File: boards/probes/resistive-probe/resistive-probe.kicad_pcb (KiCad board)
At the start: 2 copper layers, 60.5 x 6 mm, 13 parts, among them P1 MMCX, P2 SOLDERPAD, P3 SOLDERPAD

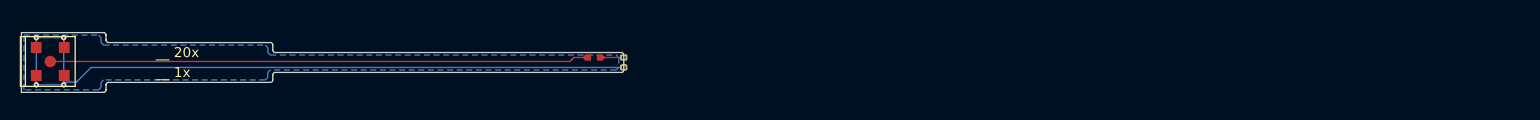
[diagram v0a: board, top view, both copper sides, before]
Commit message: v0.3 AKL-PT2 layout
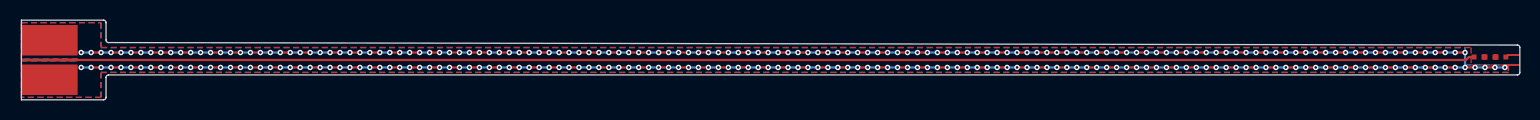
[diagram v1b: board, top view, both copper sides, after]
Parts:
- removed G*** (x4): TEARDROP_03, azonenberg_pcb:TEARDROP_03
- removed G*** (x4): TEARDROP_02, azonenberg_pcb:TEARDROP_02
- removed G***: LOGO, w_logo:Logo_silk_ROHS_5x2.8mm
- removed P1: MMCX, azonenberg_pcb:CONN_MMCX_LINX_CONNMMCX002SMD
- removed P2, P3: SOLDERPAD, azonenberg_pcb:FLEX_SOLDERPAD
- added J1: SMA, azonenberg_pcb:CONN_SMA_EDGE_AMPHENOL_901_10511_3, F.Cu at (89.3, 50.2)
- added J2: TIP, azonenberg_pcb:TESTPOINT_BARETRACE_150UM, F.Cu at (236.4, 49.8)
- added J3: GND, azonenberg_pcb:TESTPOINT_BARETRACE_150UM, F.Cu at (236.4, 50.8)
- added R2: 200, azonenberg_pcb:EIA_0402_RES_NOSILK_FLIPCHIP, F.Cu at (234.0, 50.0)
- added R3: 200, azonenberg_pcb:EIA_0402_RES_NOSILK_FLIPCHIP, F.Cu at (235.1, 50.0)
- R1: value R -> 50; footprint azonenberg_pcb:EIA_0402_RES_NOSILK -> azonenberg_pcb:EIA_0402_RES_NOSILK_FLIPCHIP
- moved R1 88.9 mm to (232.9, 50.0)
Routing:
- net /GND: track 75.9 -> 284.6 mm, vias 4 -> 284
- net Net-(J1-Pad1): track 54.3 -> 143.2 mm
- net Net-(R1-Pad1): track 2.40 -> 0.00 mm
- net Net-(J2-Pad1): track 0.00 -> 0.93 mm
- added copper zone on F.Cu, net /GND
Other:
- board size 60.5 x 6 mm -> 150.5 x 8 mm
- net class Default: clearance 0.137 -> 0.125; trace_width 0.137 -> 0.125; via_drill 0.2 -> 0.25
- rule trace_clearance: 0.137 -> 0.125
- rule trace_min: 0.137 -> 0.125
- rule via_min_drill: 0.2 -> 0.25
- board text added: "AKL-PT2 / A. Zonenberg / Antikernel Labs / Symbiotic EDA / v0.3 / 2020-10-04"
- board text removed: "137.3 um = 50 ohm Zo Assuming 1 oz Cu 75 um Er=3.4 polyimide"
- board text removed: "STARSHIPRAIDER Probe / A. Zonenberg / v0.2 / 2017-11-30"
- board text removed: "__ 1x"
- board text removed: "__ 20x"
